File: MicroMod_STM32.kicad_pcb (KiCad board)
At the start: 2 copper layers, 21.2 x 0.6 mm, 21 parts, among them J1 M.2, U1 STM32F405RGTx, Y1 CSTNE8M00GH5L000R0

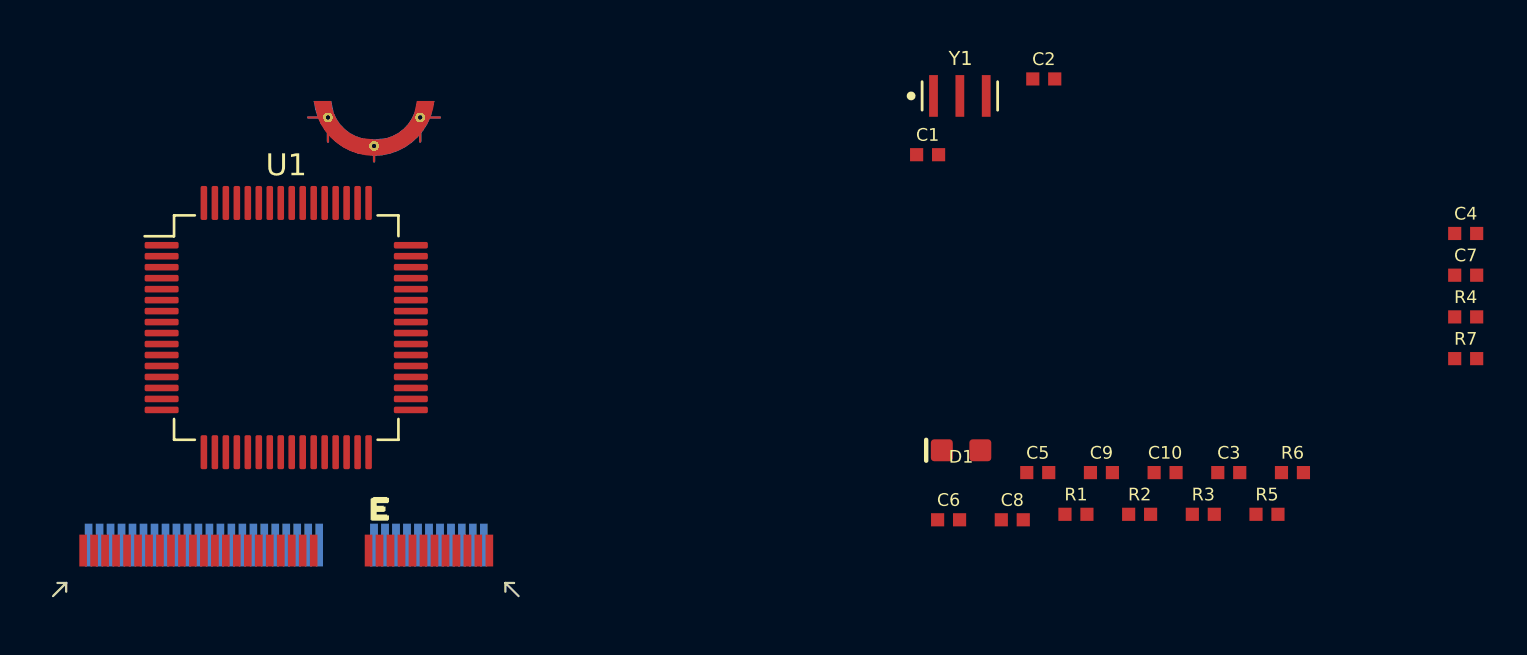
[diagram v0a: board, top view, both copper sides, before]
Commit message: update
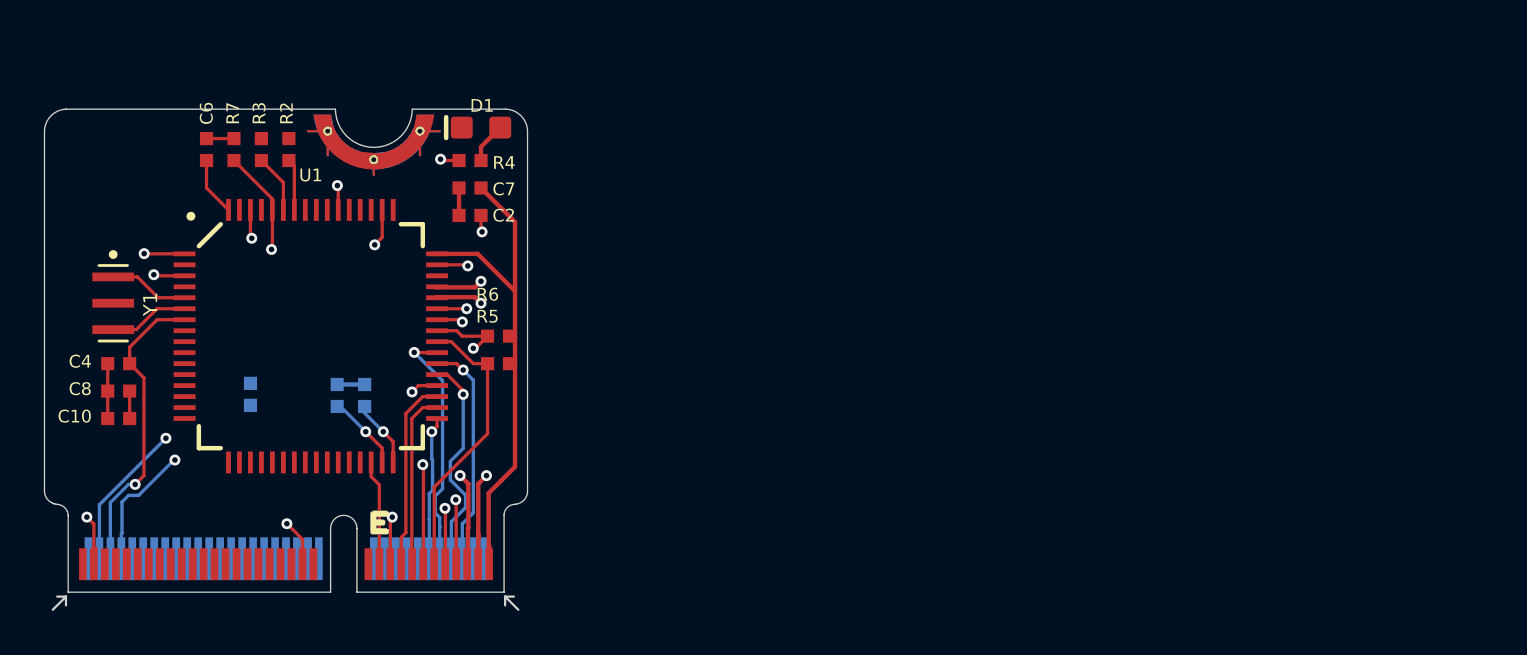
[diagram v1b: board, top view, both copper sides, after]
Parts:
- removed C3: 4.7u, MicroMod_STM32:0402-TIGHT
- removed R1: 10k, MicroMod_STM32:0402-TIGHT
- C1, C5, C9: moved to B.Cu
- U1: footprint Package_QFP:LQFP-64_10x10mm_P0.5mm -> MicroMod_STM32:TQFP64
- moved C4 61.6 mm to (48.2, 72.0)
- moved R7 56.9 mm to (53.5, 62.2), turned to 270 degrees
- moved C10 47.7 mm to (48.2, 74.5), turned to 180 degrees
- moved R3 46.0 mm to (54.8, 62.2), turned to 270 degrees
- moved R4 45.9 mm to (64.2, 62.8), turned to 180 degrees
- moved C7 45.5 mm to (64.2, 64.0), turned to 180 degrees
- moved R2 42.2 mm to (56.0, 62.2), turned to 270 degrees
- moved C8 41.1 mm to (48.2, 73.2), turned to 180 degrees
- moved Y1 39.7 mm to (48.0, 69.2), turned to 270 degrees
- moved C6 37.8 mm to (52.2, 62.2), turned to 90 degrees
- moved R6 36.7 mm to (65.5, 70.8), turned to 180 degrees
- moved C5 36.0 mm to (54.2, 73.4), turned to 90 degrees
- moved R5 35.7 mm to (65.5, 72.0), turned to 180 degrees
- moved C9 33.7 mm to (59.5, 73.5), turned to 90 degrees
- moved C1 29.0 mm to (58.2, 73.5), turned to 90 degrees
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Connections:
- J1 pad 1: Net-(J1-Pad1) -> /VCC
- J1 pad 10: Net-(J1-Pad10) -> /C8
- J1 pad 11: Net-(J1-Pad11) -> /IMU_SDA
- J1 pad 12: Net-(J1-Pad12) -> /B12
- J1 pad 13: Net-(J1-Pad13) -> /IMU_SCL
- J1 pad 15: Net-(J1-Pad15) -> /SPI2_CLK
- J1 pad 17: Net-(J1-Pad17) -> /SPI2_MISO
- J1 pad 19: Net-(J1-Pad19) -> /SPI2_MOSI
- J1 pad 2: Net-(J1-Pad2) -> /VCC
- J1 pad 21: Net-(J1-Pad21) -> /MOTOR2
- J1 pad 3: Net-(J1-Pad3) -> /OTG_FS_D+
- J1 pad 33: Net-(J1-Pad33) -> GND
- J1 pad 35: Net-(J1-Pad35) -> /INT_GYR
- J1 pad 4: Net-(J1-Pad4) -> GND
- J1 pad 5: Net-(J1-Pad5) -> /OTG_FS_D-
- J1 pad 6: Net-(J1-Pad6) -> /NRF_TX
- J1 pad 68: Net-(J1-Pad68) -> /BOOT0
- J1 pad 7: Net-(J1-Pad7) -> /OTG_FS_ID
- J1 pad 70: Net-(J1-Pad70) -> /NRST
- J1 pad 72: Net-(J1-Pad72) -> /MOTOR4
- J1 pad 73: Net-(J1-Pad73) -> /VBAT
- J1 pad 74: Net-(J1-Pad74) -> GND
- J1 pad 75: Net-(J1-Pad75) -> /VCC
- J1 pad 8: Net-(J1-Pad8) -> /NRF_RX
- J1 pad 9: Net-(J1-Pad9) -> /OTG_FS_VBUS
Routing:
- net /VCC: track 0.00 -> 29.6 mm, vias 0 -> 1
- net /BOOT0: track 0.00 -> 21.9 mm, vias 0 -> 2
- net /INT_GYR: track 0.00 -> 19.5 mm, vias 0 -> 2
- net /MOTOR4: track 0.00 -> 18.8 mm, vias 0 -> 2
- net /VBAT: track 0.00 -> 18.0 mm, vias 0 -> 2
- net /OTG_FS_D+: track 0.00 -> 15.9 mm, vias 0 -> 2
- net /MOTOR3: track 0.00 -> 15.1 mm, vias 0 -> 1
- net /OTG_FS_D-: track 0.00 -> 14.9 mm, vias 0 -> 2
- net /OTG_FS_ID: track 0.00 -> 14.3 mm, vias 0 -> 2
- net /NRST: track 0.00 -> 13.8 mm, vias 0 -> 1
- net /IMU_SCL: track 0.00 -> 13.5 mm, vias 0 -> 2
- net /OTG_FS_VBUS: track 0.00 -> 12.9 mm, vias 0 -> 2
- net /IMU_SDA: track 0.00 -> 12.9 mm
- net /C8: track 0.00 -> 11.3 mm, vias 0 -> 1
- net /NRF_TX: track 0.00 -> 10.3 mm, vias 0 -> 1
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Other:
- board size 21.2 x 0.6 mm -> 22 x 22 mm
- copper layers 2 -> 4
- net class Default: clearance 0.2 -> 0.12; trace_width 0.25 -> 0.2
- rule trace_clearance: 0.2 -> 0.12
- rule trace_min: 0.2 -> 0.15
